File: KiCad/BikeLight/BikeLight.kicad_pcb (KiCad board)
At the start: 2 copper layers, 29 parts, among them J1 Conn-01x02_P2.5mm_S2B-XH-A-BK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, J2 TYPE-C-31-M-12, J3 Conn-01x02_P2.5mm_S2B-XH-A-BK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, SW1 CK_KMS2xxG, U1 HT-CT62, U2 MPU-6050, U3 MCP1826S-33, U4 MAX17048, U5 TP4056-42-ESOP8

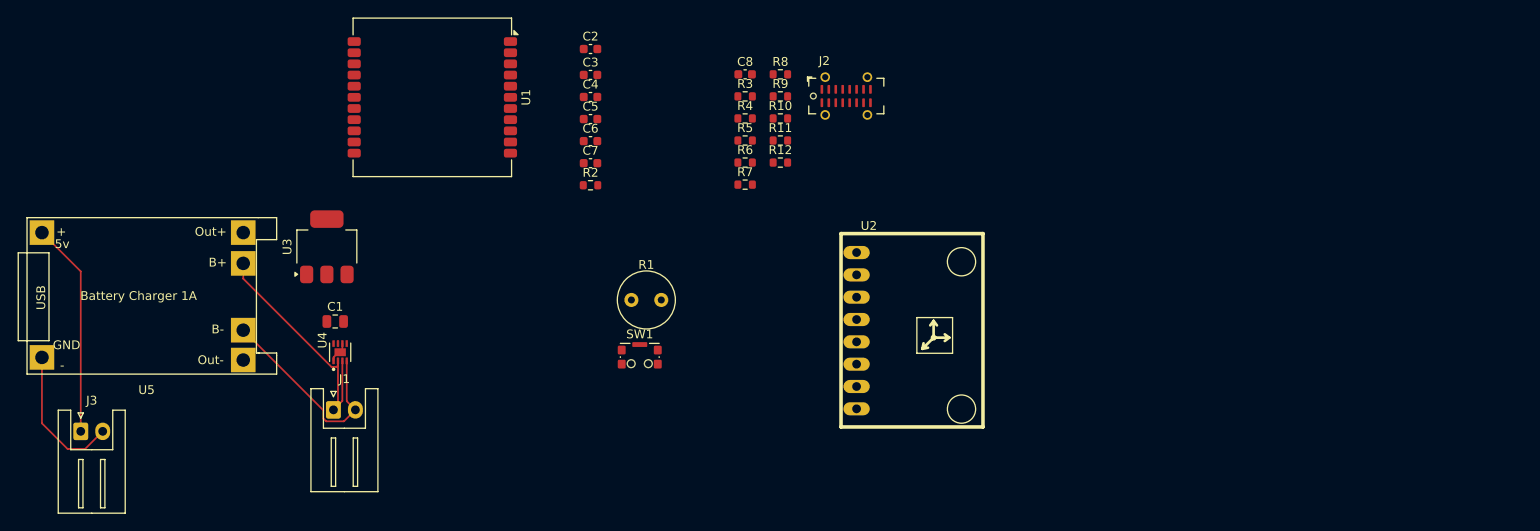
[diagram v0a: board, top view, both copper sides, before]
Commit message: Finished most of the PCB
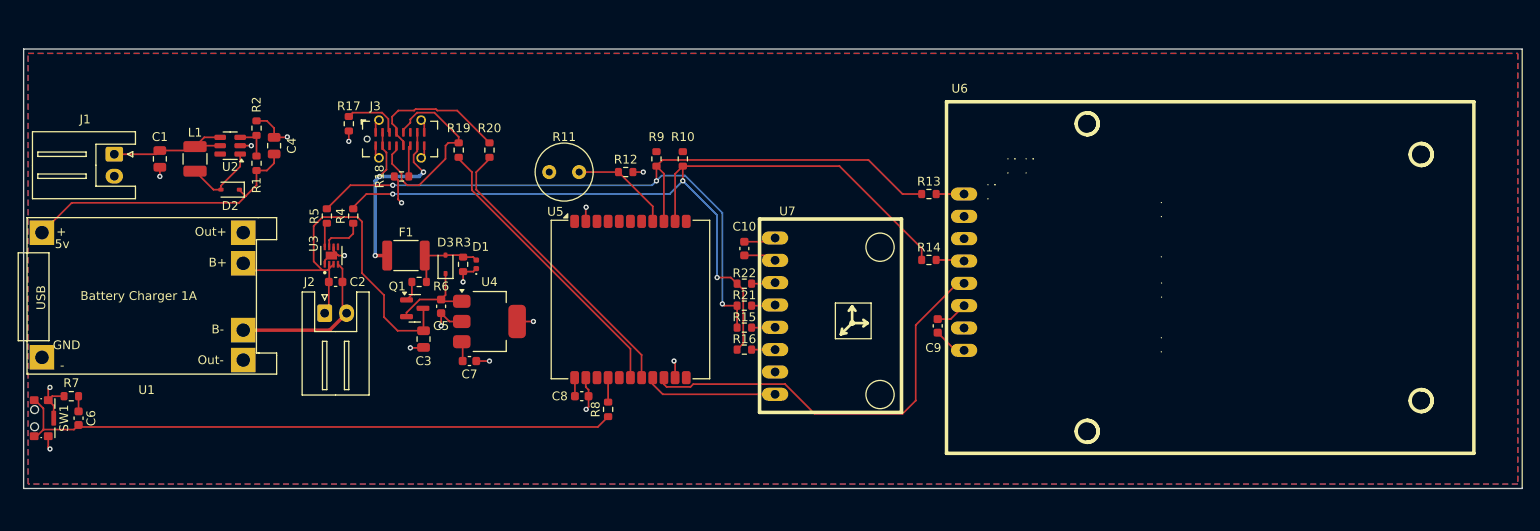
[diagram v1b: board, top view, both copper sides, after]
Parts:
- added C1: 22u_0805_CL21A226MAQNNNE, Capacitor_SMD:C_0805_2012Metric, F.Cu at (100.0, 72.5)
- added C5: 1u_0603_CL10A105KA8NNNC, Capacitor_SMD:C_0603_1608Metric, F.Cu at (132.0, 89.3)
- added D1: SOD-882_0402_RCLAMP0521P-N, Diode_SMD:D_0402_1005Metric, F.Cu at (136.0, 84.5)
- added D2: 1N5819WS, Diode_SMD:D_SOD-323, F.Cu at (108.0, 76.0)
- added D3: 1N5819WS, Diode_SMD:D_SOD-323, F.Cu at (132.5, 84.5)
- added F1: MF-MSMF010-2, Fuse:Fuse_1812_4532Metric, F.Cu at (128.0, 83.5)
- added L1: 22u_620mA_1210_CBC3225T220KR, Inductor_SMD:L_1210_3225Metric, F.Cu at (104.0, 72.5)
- added Q1: AO3401A, Package_TO_SOT_SMD:SOT-23, F.Cu at (129.0, 89.5)
- added R1: 47k_0402_0402WGF1002TCE, Resistor_SMD:R_0603_1608Metric, F.Cu at (111.0, 73.0)
- added R17: 5.1k_0603_0603WAF5101T5E, Resistor_SMD:R_0603_1608Metric, F.Cu at (121.5, 68.5)
- added R18: 5.1k_0603_0603WAF5101T5E, Resistor_SMD:R_0603_1608Metric, F.Cu at (127.5, 74.5)
- added R19: 0R_0603_0603WAF0000T5E, Resistor_SMD:R_0603_1608Metric, F.Cu at (134.0, 71.5)
- added R2: 10k_0603_RC0603JR-0710KL, Resistor_SMD:R_0603_1608Metric, F.Cu at (111.0, 69.0)
- added R20: 0R_0603_0603WAF0000T5E, Resistor_SMD:R_0603_1608Metric, F.Cu at (137.5, 71.5)
- added R21: 0R_0603_0603WAF0000T5E, Resistor_SMD:R_0603_1608Metric, F.Cu at (166.5, 89.2)
- added R22: 0R_0603_0603WAF0000T5E, Resistor_SMD:R_0603_1608Metric, F.Cu at (166.5, 86.7)
- added R3: 10k_0603_RC0603JR-0710KL, Resistor_SMD:R_0603_1608Metric, F.Cu at (134.5, 84.5)
- added R6: 1k_0603_RMC06031K1%N, Resistor_SMD:R_0603_1608Metric, F.Cu at (129.5, 86.5)
- added U2: MT3608, Package_TO_SOT_SMD:SOT-23-6, F.Cu at (108.0, 71.0)
- added U6: RFID-RC522, Personal_Library:RFID_RC522, F.Cu at (191.5, 76.5)
- C4: value 100n_0603_TCC0603X7R104K500CT -> 22u_0805_CL21A226MAQNNNE; footprint Capacitor_SMD:C_0603_1608Metric -> Capacitor_SMD:C_0805_2012Metric
- J3: renamed from J2; value TYPE-C-31-M-12 -> GT-USB-7051A
- moved SW1 68.5 mm to (86.5, 102.0), turned to -90 degrees
- moved C6 66.2 mm to (90.8, 102.0), turned to -90 degrees
- moved R7 63.8 mm to (89.9, 99.5), turned to 180 degrees
- moved R4 51.2 mm to (122.0, 79.0), turned to 90 degrees
- moved J3 51.0 mm to (127.3, 70.2)
- moved R5 47.7 mm to (119.0, 79.0), turned to 90 degrees
- moved C7 38.1 mm to (135.2, 95.5)
- moved C8 36.6 mm to (148.0, 99.5)
- moved C4 36.4 mm to (113.0, 71.0), turned to 90 degrees
- moved C9 36.0 mm to (188.5, 91.5), turned to 90 degrees
- moved R8 34.3 mm to (151.0, 101.0), turned to 90 degrees
- moved U5 32.2 mm to (153.5, 88.5), turned to 0 degrees
- moved C2 32.0 mm to (120.0, 86.5)
- moved J1 31.8 mm to (94.8, 72.0), turned to -90 degrees
- moved R14 23.3 mm to (187.5, 84.0)
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- renumbered C5 to C10, C7 to C2, C1 to C3, C2 to C7, C3 to C8, C8 to C9, J3 to J1, J1 to J2, R4 to R10, R1 to R11, R6 to R12, R9 to R13, R10 to R14, R11 to R15, R12 to R16, R8 to R4, R7 to R5, R2 to R7, R5 to R8, R3 to R9, U5 to U1, U4 to U3, U3 to U4, U1 to U5, U2 to U7
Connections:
- net Net-(J2-VBUS-PadA4) renamed VBUS
- C4 pad 1: GND -> VSOL
- J1 pad 1: Net-(J3-Pin_1) -> +SOLAR
- J1 pad 2: Net-(J3-Pin_2) -> GND
- J3 pad A1: Net-(J2-GND-PadA1) -> GND
- J3 pad A12: Net-(J2-GND-PadA1) -> GND
- J3 pad A5: unconnected-(J2-CC1-PadA5) -> Net-(J3-CC1)
- J3 pad A6: unconnected-(J2-D+-PadA6) -> Net-(J3-D+-PadA6)
- J3 pad A7: unconnected-(J2-D--PadA7) -> Net-(J3-D--PadA7)
- J3 pad B1: Net-(J2-GND-PadA1) -> GND
- J3 pad B12: Net-(J2-GND-PadA1) -> GND
- J3 pad B5: unconnected-(J2-CC2-PadB5) -> Net-(J3-CC2)
- J3 pad B6: unconnected-(J2-D+-PadB6) -> Net-(J3-D+-PadA6)
- J3 pad B7: unconnected-(J2-D--PadB7) -> Net-(J3-D--PadA7)
- J3 pad S1: unconnected-(J2-SHIELD-PadS1) -> GND
- R5 pad 1: /SDA -> Net-(U3-SDA)
- R5 pad 2: Net-(U4-SDA) -> /SDA
- U1 pad 1: Net-(J3-Pin_1) -> VSOL
- U1 pad 2: Net-(J3-Pin_2) -> GND
- U3 pad 8: Net-(U4-SDA) -> Net-(U3-SDA)
- U4 pad 1: +BATT -> Net-(D3-K)
- U5 pad 17: unconnected-(U1-GPIO18_DN-Pad17) -> /USB_DN
- U5 pad 18: unconnected-(U1-GPIO19_DP-Pad18) -> /USB_DP
- U5 pad 19: unconnected-(U1-GPIO20_RXD-Pad19) -> /ACC_INT
- U7 pad 3: unconnected-(U2-SCL-Pad3) -> Net-(U7-SCL)
- U7 pad 4: unconnected-(U2-SDA-Pad4) -> Net-(U7-SDA)
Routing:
- net /SDA: track 0.00 -> 103.3 mm, vias 0 -> 3
- net /SCL: track 0.00 -> 102.9 mm, vias 0 -> 3
- net Net-(C6-Pad2): track 0.00 -> 70.3 mm
- net GND: track 2.49 -> 57.5 mm, vias 0 -> 17
- net /IRQ_RFID: track 0.00 -> 47.7 mm
- net /USB_DP: track 0.00 -> 33.5 mm
- net /USB_DN: track 0.00 -> 33.2 mm
- net VSOL: track 0.00 -> 32.8 mm
- net VBUS: track 0.00 -> 26.5 mm, vias 0 -> 3
- net Net-(J3-Pin_1): track 24.4 -> 0.00 mm
- net Net-(J3-D--PadA7): track 0.00 -> 23.6 mm
- net +BATT: track 29.0 -> 48.6 mm
- net Net-(J3-D+-PadA6): track 0.00 -> 16.8 mm
- net Net-(J3-Pin_2): track 16.4 -> 0.00 mm
- net +SOLAR: track 0.00 -> 15.7 mm
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- added copper zone on F.Cu, net +3.3V
- added copper zone on B.Cu, net GND
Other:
- board outline added: 170.5 x 50 mm
